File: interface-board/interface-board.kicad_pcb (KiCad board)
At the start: 2 copper layers, 181.5 x 110 mm, 97 parts, among them J1 HECS, J10 AUX, J11 UART, J12 NTC1, J13 NTC1, J15 ICSP, J16 Conn_01x23, J2 CASEFAN1, J3 CASEFAN2, J4 Bender-LV, J6 HV+, J7 HV-, J8 IMD, J9 TSMP, Q1 Q_NMOS_GDS, Q2 Q_NMOS_GDS, Q3 Q_NMOS_GDS, Q4 Q_NMOS_GDS, U1 MCP2551-I-SN, U2 MCP2515-IST, U3 ATmega328P-AU, U4 LTV-827S, U5 DCM4623TD2J13D0T70, U6 LTV-824, U7 R-78E5.0-0.5, U8 INA219, Y1 16MHz

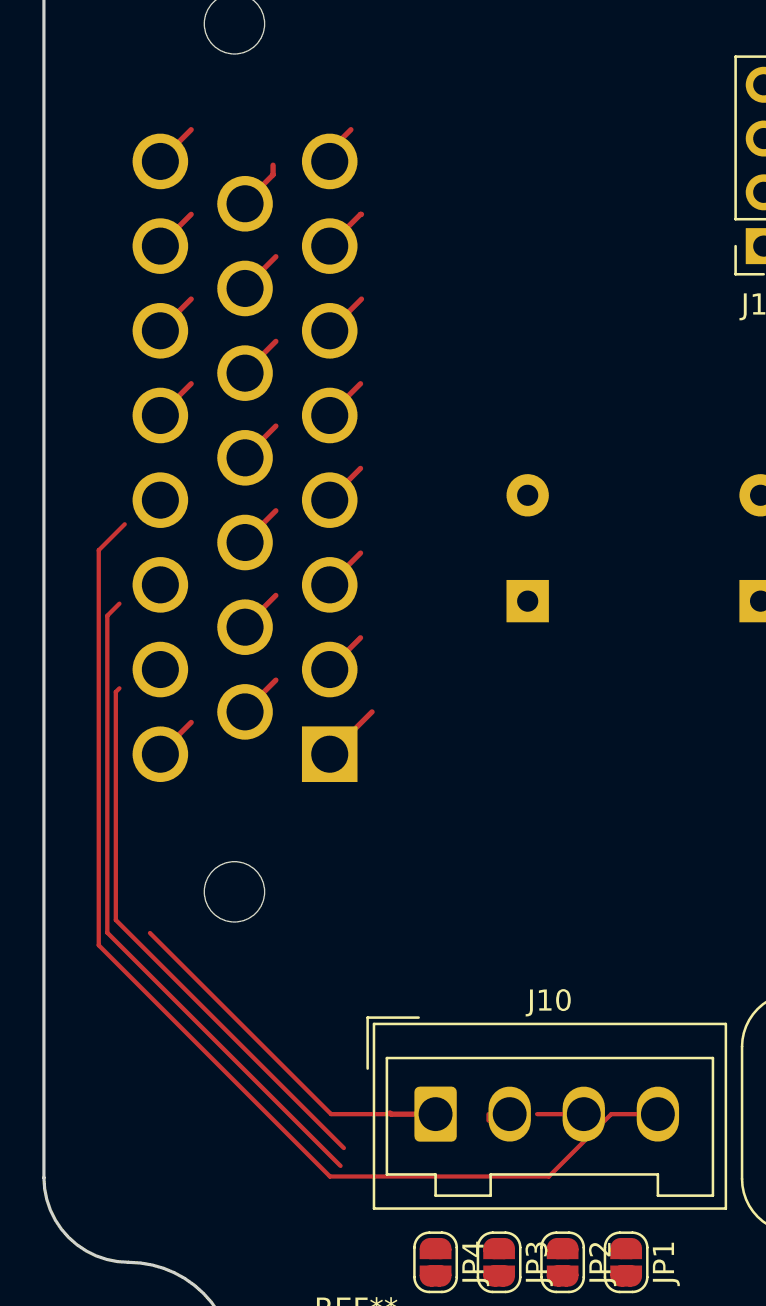
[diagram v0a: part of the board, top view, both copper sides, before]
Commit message: Fixed more shit
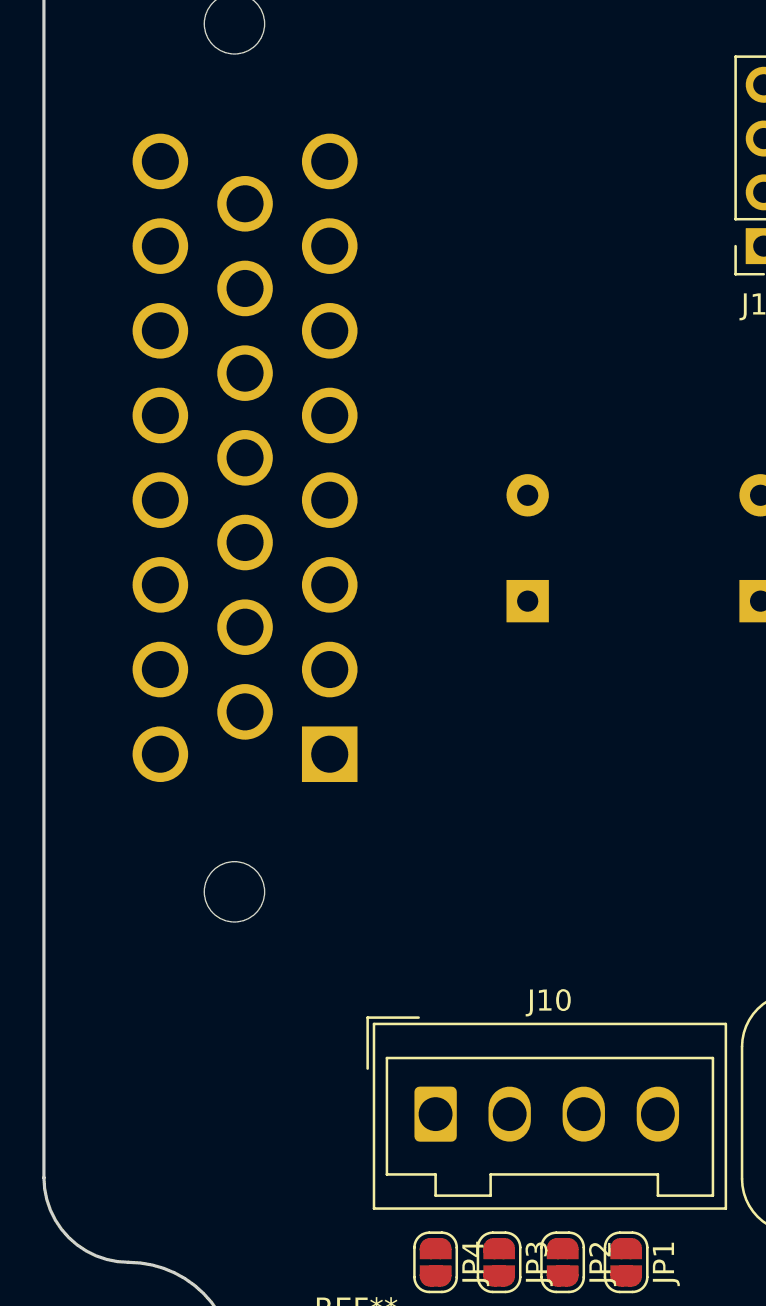
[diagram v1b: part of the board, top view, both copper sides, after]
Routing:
- net (no net): track 51.5 -> 0.00 mm
- net Net-(J10-Pad3): track 32.6 -> 0.00 mm
- net Net-(J10-Pad2): track 26.5 -> 0.00 mm
- net Net-(J10-Pad1): track 17.2 -> 0.00 mm
- net /SHDN_LOOP_OUT: track 11.0 -> 0.00 mm
- net GND: track 8.17 -> 0.00 mm
- net +12V: track 4.13 -> 0.00 mm
- net /FANOUT2: track 2.31 -> 0.00 mm
- net /FANOUT3: track 2.09 -> 0.00 mm
- net /IMD_AN3: track 2.04 -> 0.00 mm
- net /IMD_AN2: track 2.04 -> 0.00 mm
- net /IMD_AN1: track 2.04 -> 0.00 mm
- net /CAN-: track 2.04 -> 0.00 mm
- net /CAN+: track 2.04 -> 0.00 mm
- net +5V: track 2.04 -> 0.00 mm
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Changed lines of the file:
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@@
-(kicad_pcb (version 20171130) (host pcbnew "(5.0.0)")
+(kicad_pcb (version 20171130) (host pcbnew "(5.0.2)-1")
   (general
     (thickness 1.6)
     (drawings 60)
-    (tracks 43)
+    (tracks 0)
     (zones 0)
     (modules 97)
@@
   (gr_line (start 119 -61) (end 119 43) (layer Edge.Cuts) (width 0.15))
   (gr_line (start 116 -64) (end -50.5 -64) (layer Edge.Cuts) (width 0.15))
-  (segment (start -35.7032 21.5) (end -38.6482 24.445) (width 0.2032) (layer F.Cu) (net 0))
-  (segment (start -34.5 21.5) (end -35.7032 21.5) (width 0.2032) (layer F.Cu) (net 0) (status 10))
-  (segment (start -38.6482 24.445) (end -48.99 24.445) (width 0.2032) (layer F.Cu) (net 0))
-  (segment (start -59.910522 13.524478) (end -59.910522 -5.134478) (width 0.2032) (layer F.Cu) (net 0))
-  (segment (start -48.99 24.445) (end -59.910522 13.524478) (width 0.2032) (layer F.Cu) (net 0))
-  (segment (start -59.910522 -5.134478) (end -58.684435 -6.360565) (width 0.2032) (layer F.Cu) (net 0))
-  (segment (start -48.99 -15.555) (end -48.945 -15.555) (width 0.25) (layer F.Cu) (net 1) (status 30))
-  (segment (start -48.945 -15.555) (end -47.5 -17) (width 0.25) (layer F.Cu) (net 1) (status 10))
-  (segment (start -52.99 -17.555) (end -51.545 -19) (width 0.25) (layer F.Cu) (net 1) (status 10))
-  (segment (start -48.99 -3.555) (end -47.545 -5) (width 0.25) (layer F.Cu) (net 2) (status 10))
-  (segment (start -48.99 -7.555) (end -47.545 -9) (width 0.25) (layer F.Cu) (net 2) (status 10))
-  (segment (start -48.99 -11.555) (end -47.545 -13) (width 0.25) (layer F.Cu) (net 2) (status 10))
-  (segment (start -52.99 -13.555) (end -51.545 -15) (width 0.25) (layer F.Cu) (net 2) (status 10))
-  (segment (start -56.99 -23.555) (end -55.545 -25) (width 0.25) (layer F.Cu) (net 3) (status 10))
-  (segment (start -51.677501 -22.867499) (end -51.677501 -23.322499) (width 0.25) (layer F.Cu) (net 18))
-  (segment (start -52.99 -21.555) (end -51.677501 -22.867499) (width 0.25) (layer F.Cu) (net 18) (status 10))
-  (segment (start -48.99 -23.555) (end -48.99 -24.01) (width 0.25) (layer F.Cu) (net 19) (status 30))
-  (segment (start -48.99 -24.01) (end -48 -25) (width 0.25) (layer F.Cu) (net 19) (status 10))
-  (segment (start -48.99 -19.555) (end -47.545 -21) (width 0.25) (layer F.Cu) (net 20) (status 10))
-  (segment (start -47.545 -21) (end -47.5 -21) (width 0.25) (layer F.Cu) (net 20))
-  (segment (start -56.99 -19.555) (end -55.545 -21) (width 0.25) (layer F.Cu) (net 23) (status 10))
-  (segment (start -56.99 -15.555) (end -55.545 -17) (width 0.25) (layer F.Cu) (net 24) (status 10))
-  (segment (start -56.99 -11.555) (end -55.545 -13) (width 0.25) (layer F.Cu) (net 25) (status 10))
-  (segment (start -46.1 21.5) (end -46.155 21.445) (width 0.25) (layer F.Cu) (net 26))
-  (segment (start -45 21.5) (end -46.1 21.5) (width 0.25) (layer F.Cu) (net 26) (status 10))
-  (segment (start -45 21.5) (end -48.935 21.5) (width 0.2032) (layer F.Cu) (net 26) (status 10))
-  (segment (start -48.935 21.5) (end -57.49 12.945) (width 0.2032) (layer F.Cu) (net 26))
-  (segment (start -41.5 21.5) (end -41.5 21.8) (width 0.2032) (layer F.Cu) (net 27) (status 30))
-  (segment (start -59.104101 12.330899) (end -59.104101 1.559101) (width 0.2032) (layer F.Cu) (net 27))
-  (segment (start -48.33339 23.10161) (end -59.104101 12.330899) (width 0.2032) (layer F.Cu) (net 27))
-  (segment (start -59.104101 1.559101) (end -58.934435 1.389435) (width 0.2032) (layer F.Cu) (net 27))
-  (segment (start -38 21.5) (end -39.2032 21.5) (width 0.2032) (layer F.Cu) (net 28) (status 10))
-  (segment (start -59.507316 12.927683) (end -59.507316 -2.037684) (width 0.2032) (layer F.Cu) (net 28))
-  (segment (start -48.49 23.945) (end -59.507316 12.927683) (width 0.2032) (layer F.Cu) (net 28))
-  (segment (start -59.507316 -2.037684) (end -58.934435 -2.610565) (width 0.2032) (layer F.Cu) (net 28))
-  (segment (start -52.99 -9.555) (end -51.545 -11) (width 0.25) (layer F.Cu) (net 29) (status 10))
-  (segment (start -52.99 -5.555) (end -51.545 -7) (width 0.25) (layer F.Cu) (net 30) (status 10))
-  (segment (start -56.99 4.445) (end -55.545 3) (width 0.25) (layer F.Cu) (net 39) (status 10))
-  (segment (start -52.99 2.445) (end -51.545 1) (width 0.25) (layer F.Cu) (net 39) (status 10))
-  (segment (start -48.99 4.445) (end -48.945 4.445) (width 0.25) (layer F.Cu) (net 39) (status 30))
-  (segment (start -48.945 4.445) (end -47 2.5) (width 0.25) (layer F.Cu) (net 39) (status 10))
-  (segment (start -48.99 0.445) (end -47.545 -1) (width 0.25) (layer F.Cu) (net 39) (status 10))
-  (segment (start -52.99 -1.555) (end -51.545 -3) (width 0.25) (layer F.Cu) (net 39) (status 10))
 )
